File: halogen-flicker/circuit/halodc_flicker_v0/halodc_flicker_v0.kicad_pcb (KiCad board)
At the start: 2 copper layers, 86.1 x 45.6 mm, 21 parts, among them J1 ASP, J2 BATT_LAMP, J4 CHARGER, Q1 IRF540N, SW1 SW_DIP_x02, SW2 SW_Push, U1 ATtiny13A-S, U2 PC817, U3 AMS1117-5.0

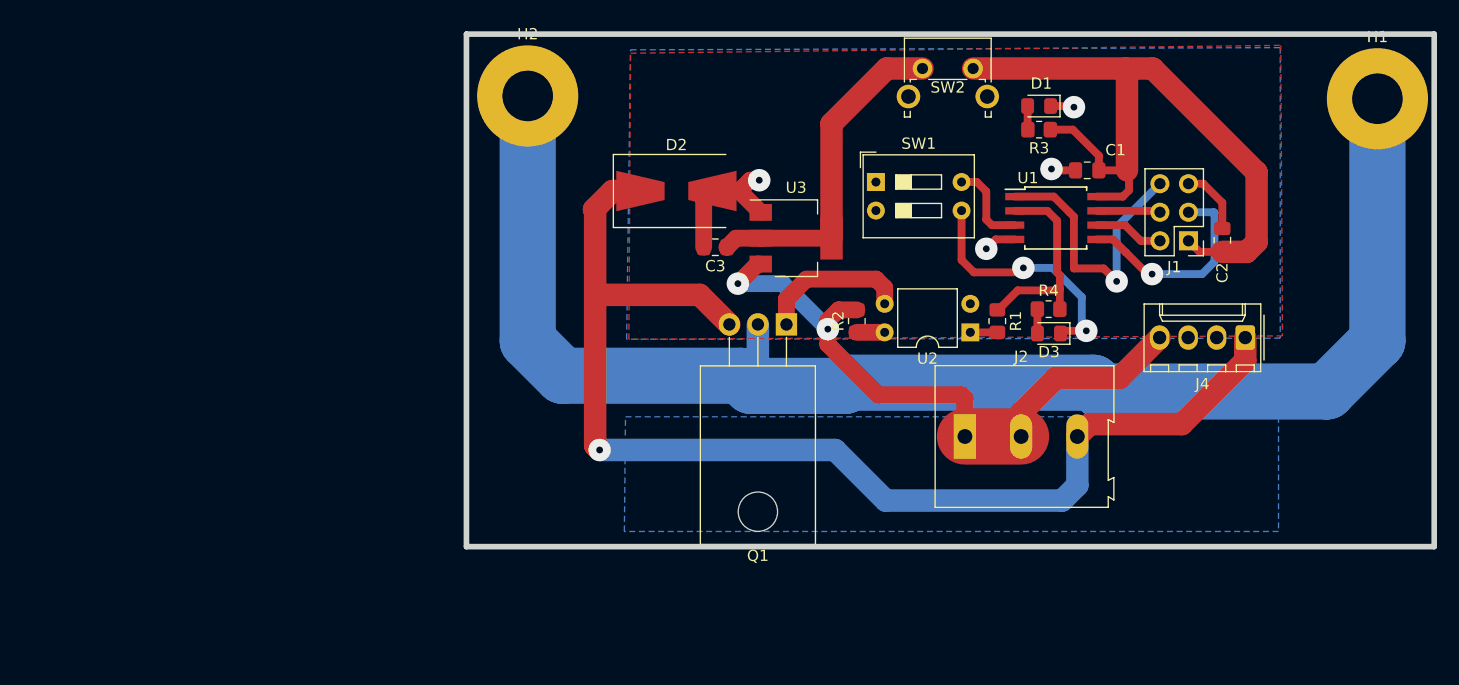
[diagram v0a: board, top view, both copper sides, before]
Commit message: Halogen Flicker
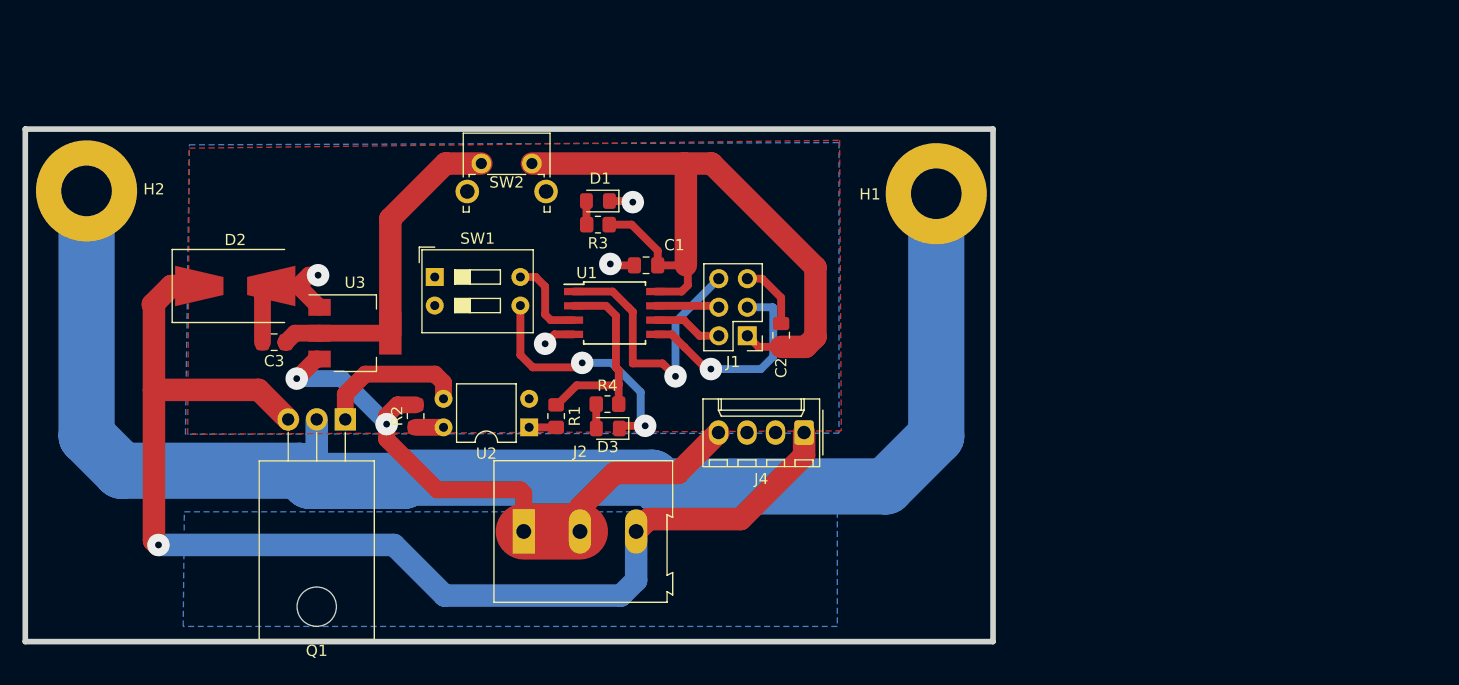
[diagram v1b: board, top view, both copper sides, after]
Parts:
- moved Q1 40.1 mm to (101.8, 65.3)
- moved C1 40.1 mm to (128.5, 51.6)
- moved C2 40.1 mm to (140.6, 57.8)
- moved C3 40.1 mm to (95.4, 58.4)
- moved D1 40.1 mm to (124.2, 45.9)
- moved D3 40.1 mm to (125.1, 66.1)
- moved H1 40.1 mm to (154.3, 45.2)
- moved H2 40.1 mm to (78.8, 45.0)
- moved J1 40.1 mm to (137.5, 57.8)
- moved J2 40.1 mm to (117.7, 75.2)
- moved J4 40.1 mm to (142.6, 66.5)
- moved R1 40.1 mm to (120.5, 65.0)
- moved R2 40.1 mm to (108.0, 65.0)
- moved R3 40.1 mm to (124.2, 48.0)
- moved R4 40.1 mm to (125.1, 63.9)
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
